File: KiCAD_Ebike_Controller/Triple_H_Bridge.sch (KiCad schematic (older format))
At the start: 24 parts, among them Q1 DMT10H010LK3, Q2 DMT10H010LK3, Q3 DMT10H010LK3, Q4 DMT10H010LK3, Q5 DMT10H010LK3, Q6 DMT10H010LK3

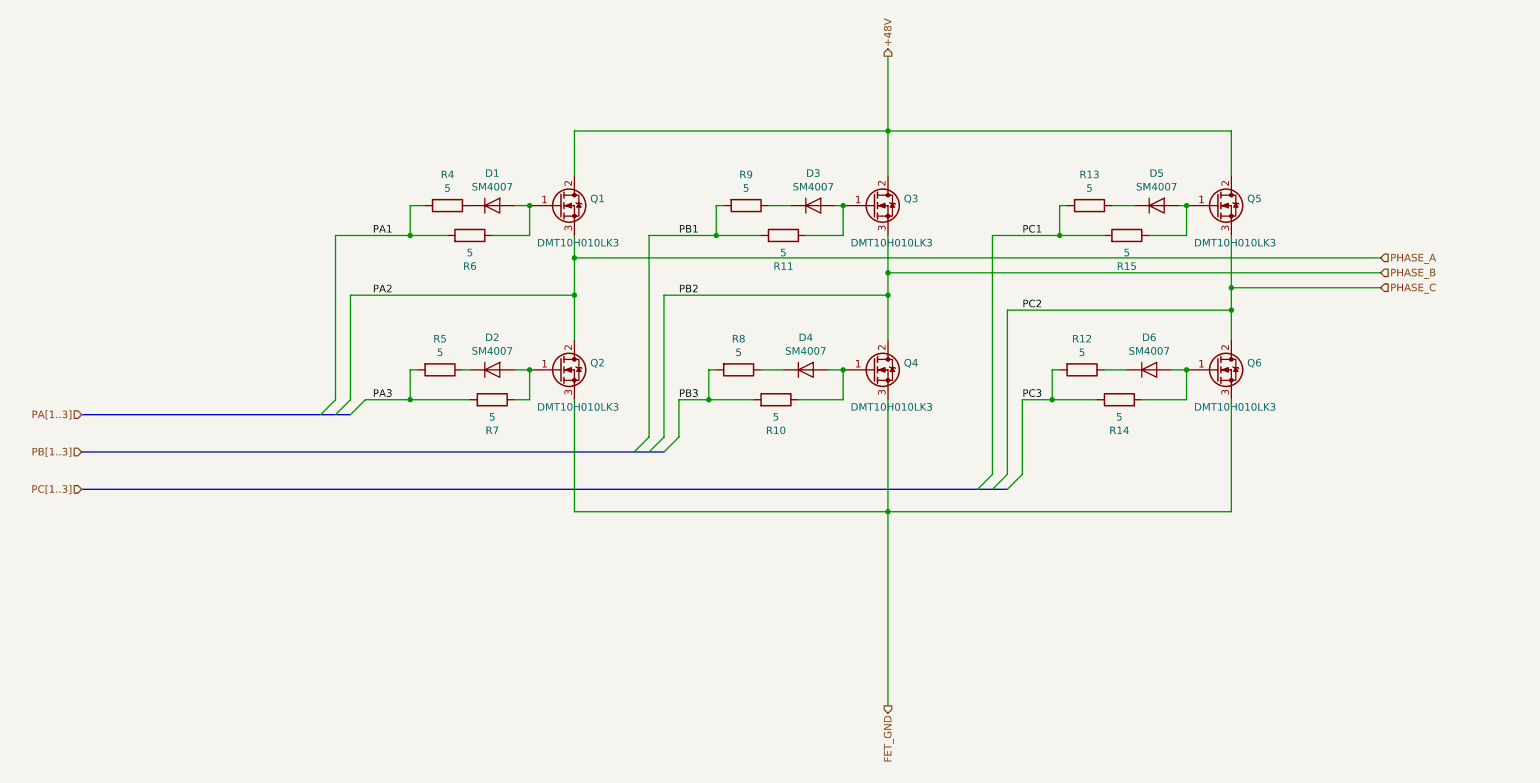
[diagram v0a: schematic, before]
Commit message: Finished ready for fab
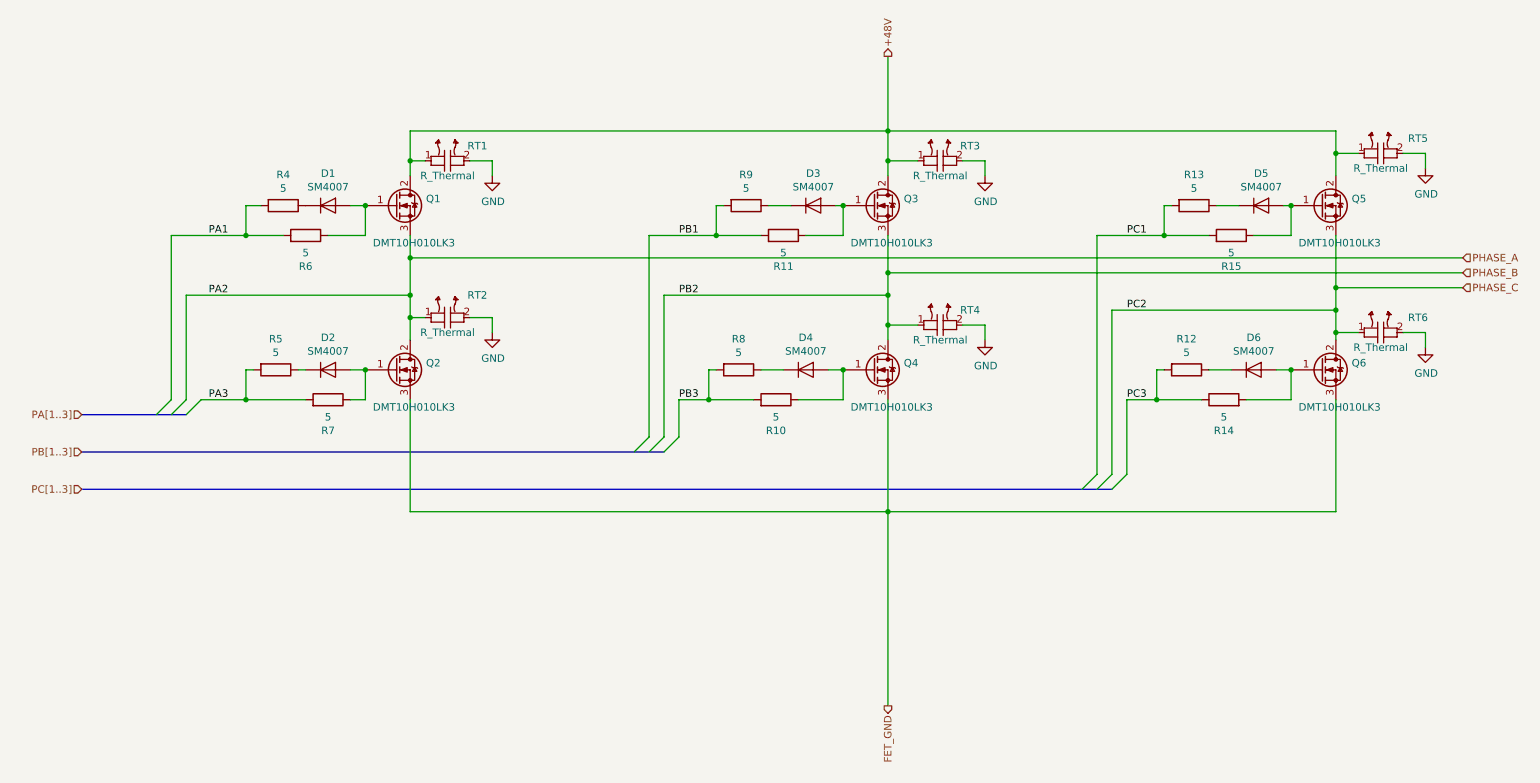
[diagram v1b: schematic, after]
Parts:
- added RT1, RT2, RT3, RT4, RT5, RT6: R_Thermal, Resistor_SMD:R_1206_3216Metric_Pad1.42x1.75mm_HandSolder, symbol Device:R_Thermal
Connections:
- net +48V: now also RT1.1, RT3.1, RT5.1
- net PHASE_A: now also RT2.1
- net PHASE_B: now also RT4.1
- net PHASE_C: now also RT6.1
- new net GND: RT1.2, RT2.2, RT3.2, RT4.2, RT5.2, RT6.2
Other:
- moved on the sheet: D1, D2, D5, D6, Q1, Q2, Q5, Q6, R12, R13, R14, R15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
